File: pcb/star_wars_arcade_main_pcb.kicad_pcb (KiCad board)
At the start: 2 copper layers, 292.1 x 525.8 mm, 323 parts, among them J16 Aud_Conn, J17 Main_Connector, J18 Cat_Box_Conn, J20 J20, Q1 2N3904, Q3 Q_NPN_BCE, Q4 Q_NPN_BCE, SW1 L_11, SW2 D_10, SW3 E/F_10, Y1 12.096MHz

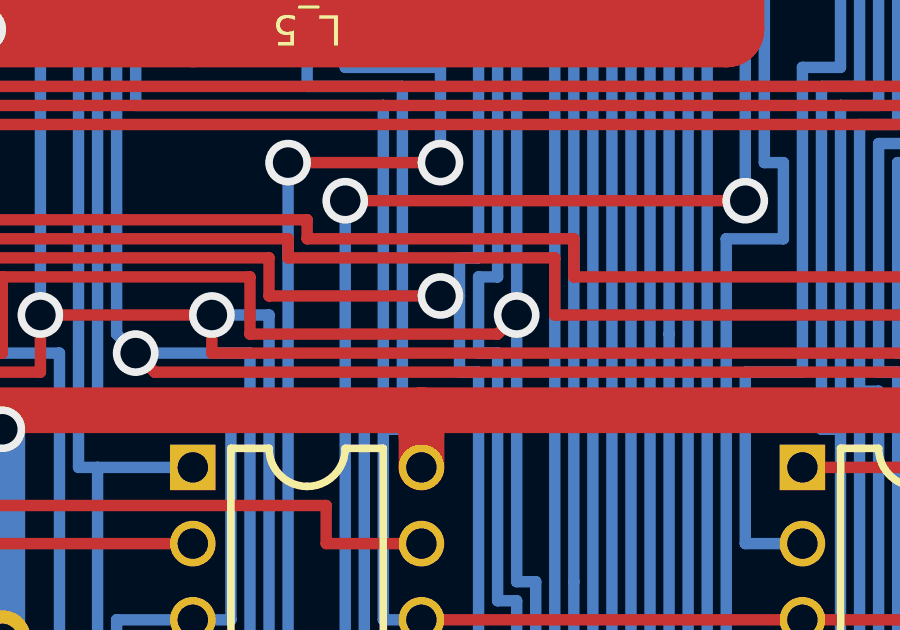
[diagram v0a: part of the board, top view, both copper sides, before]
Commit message: Updated readme file
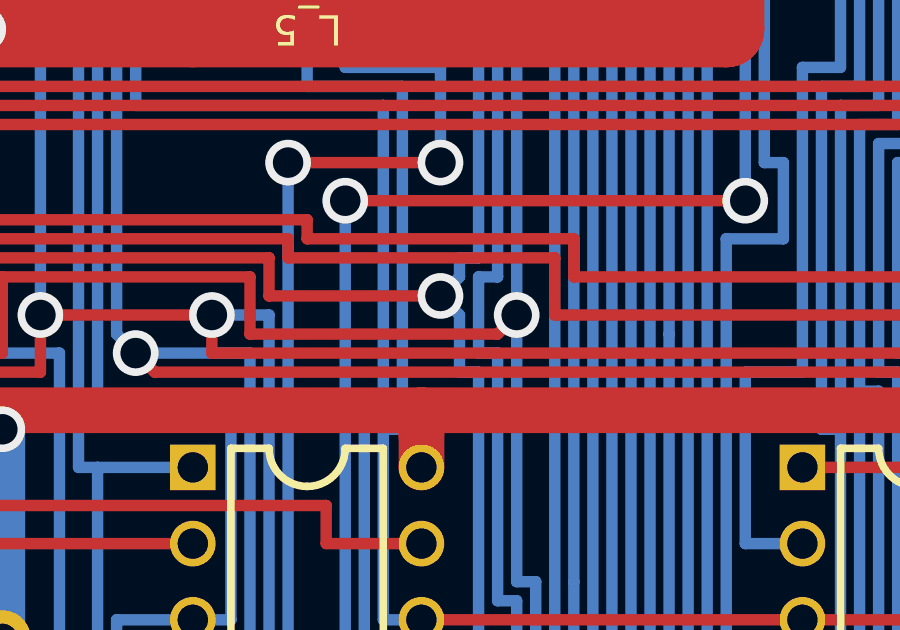
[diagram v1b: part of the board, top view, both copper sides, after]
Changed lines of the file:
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@@
     (thickness 1.6)
     (drawings 118)
-    (tracks 10588)
+    (tracks 10589)
     (zones 0)
     (modules 323)
@@
     (visible_elements 7FFFF7FF)
     (pcbplotparams
-      (layerselection 0x010fc_ffffffff)
+      (layerselection 0x010f0_ffffffff)
       (usegerberextensions false)
       (usegerberattributes false)
@@
   (segment (start 122.555 363.22) (end 124.46 363.22) (width 0.381) (layer B.Cu) (net 123))
   (segment (start 124.46 363.22) (end 124.46 359.41) (width 0.381) (layer B.Cu) (net 123))
-  (segment (start 122.555 323.215) (end 123.825 323.215) (width 0.381) (layer B.Cu) (net 123))
-  (segment (start 123.825 323.215) (end 123.825 332.74) (width 0.381) (layer B.Cu) (net 123))
-  (segment (start 123.825 332.74) (end 124.46 332.74) (width 0.381) (layer B.Cu) (net 123))
-  (segment (start 124.46 332.74) (end 124.46 340.995) (width 0.381) (layer B.Cu) (net 123))
-  (segment (start 124.46 340.995) (end 123.825 340.995) (width 0.381) (layer B.Cu) (net 123))
-  (segment (start 123.19 342.265) (end 123.825 342.265) (width 0.381) (layer B.Cu) (net 123))
-  (segment (start 123.825 340.995) (end 123.825 342.265) (width 0.381) (layer B.Cu) (net 123))
-  (segment (start 123.825 342.265) (end 123.825 344.805) (width 0.381) (layer B.Cu) (net 123))
-  (segment (start 124.46 344.805) (end 124.46 359.41) (width 0.381) (layer B.Cu) (net 123))
-  (segment (start 123.825 344.805) (end 124.46 344.805) (width 0.381) (layer B.Cu) (net 123))
   (segment (start 161.29 274.955) (end 163.83 274.955) (width 0.381) (layer B.Cu) (net 123))
   (segment (start 161.29 309.245) (end 161.29 274.955) (width 0.381) (layer B.Cu) (net 123))
@@
   (segment (start 247.015 361.95) (end 247.015 360.68) (width 0.381) (layer F.Cu) (net 123))
   (segment (start 222.885 363.22) (end 222.885 361.95) (width 0.381) (layer F.Cu) (net 123))
+  (segment (start 123.825 344.805) (end 124.46 344.805) (width 0.381) (layer B.Cu) (net 123))
+  (segment (start 123.825 323.215) (end 123.825 332.74) (width 0.381) (layer B.Cu) (net 123))
+  (segment (start 124.46 332.74) (end 124.46 340.995) (width 0.381) (layer B.Cu) (net 123))
+  (segment (start 123.825 332.74) (end 124.46 332.74) (width 0.381) (layer B.Cu) (net 123))
+  (segment (start 124.46 344.805) (end 124.46 359.41) (width 0.381) (layer B.Cu) (net 123))
+  (segment (start 122.555 323.215) (end 123.825 323.215) (width 0.381) (layer B.Cu) (net 123))
+  (segment (start 124.46 340.995) (end 123.825 340.995) (width 0.381) (layer B.Cu) (net 123))
+  (segment (start 123.825 344.805) (end 123.825 342.9) (width 0.381) (layer B.Cu) (net 123))
+  (segment (start 123.825 342.9) (end 123.19 342.265) (width 0.381) (layer B.Cu) (net 123))
+  (segment (start 123.825 340.995) (end 123.825 341.63) (width 0.381) (layer B.Cu) (net 123))
+  (segment (start 123.825 341.63) (end 123.19 342.265) (width 0.381) (layer B.Cu) (net 123))
   (segment (start 241.935 355.6) (end 229.87 355.6) (width 0.381) (layer F.Cu) (net 124))
   (segment (start 229.87 355.6) (end 229.87 355.6) (width 0.381) (layer F.Cu) (net 124))
